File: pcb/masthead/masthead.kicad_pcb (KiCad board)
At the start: 2 copper layers, 48.6 x 56.5 mm, 12 parts, among them J1 Screw_Terminal_01x01, J2 Screw_Terminal_01x01, J3 VEML7700, SW1 TILT, U1 TSR_1-2450, U2 WeMos_mini, U3 BMP581

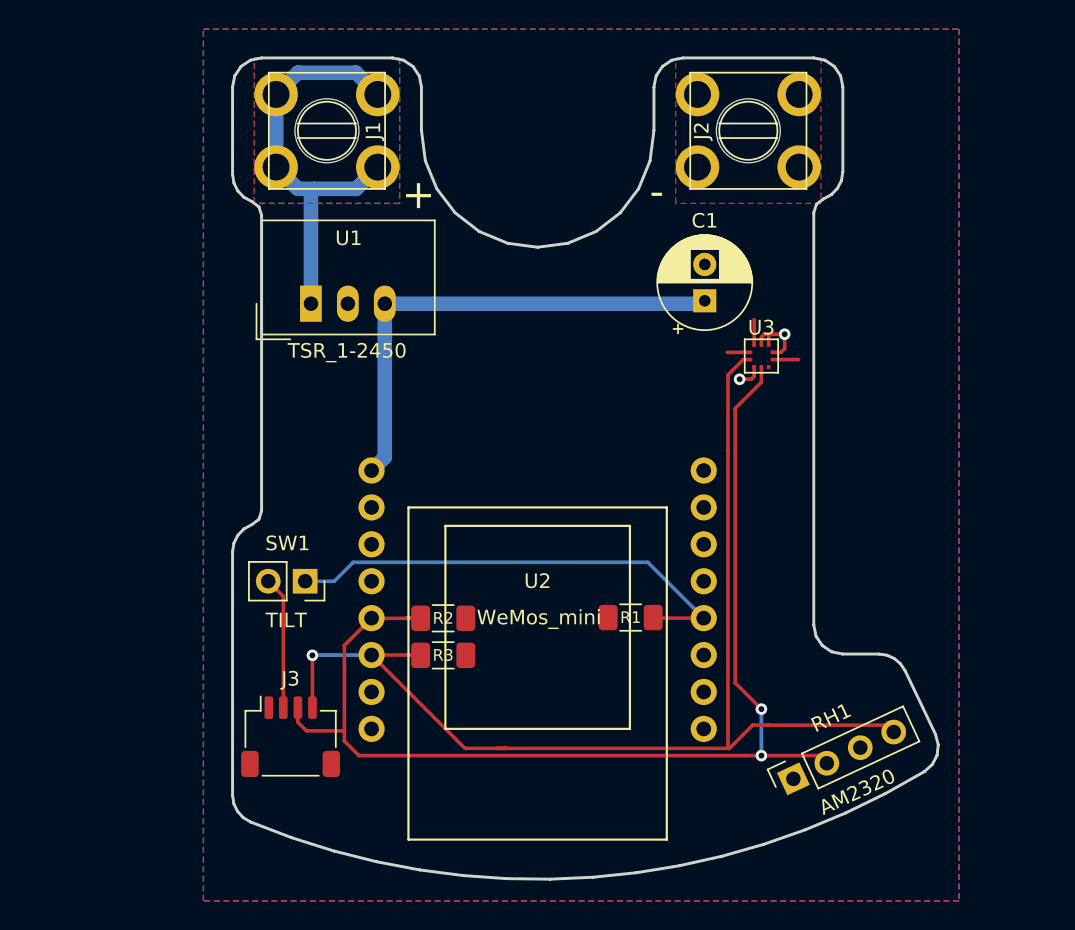
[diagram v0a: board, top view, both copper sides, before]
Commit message: Tweaks
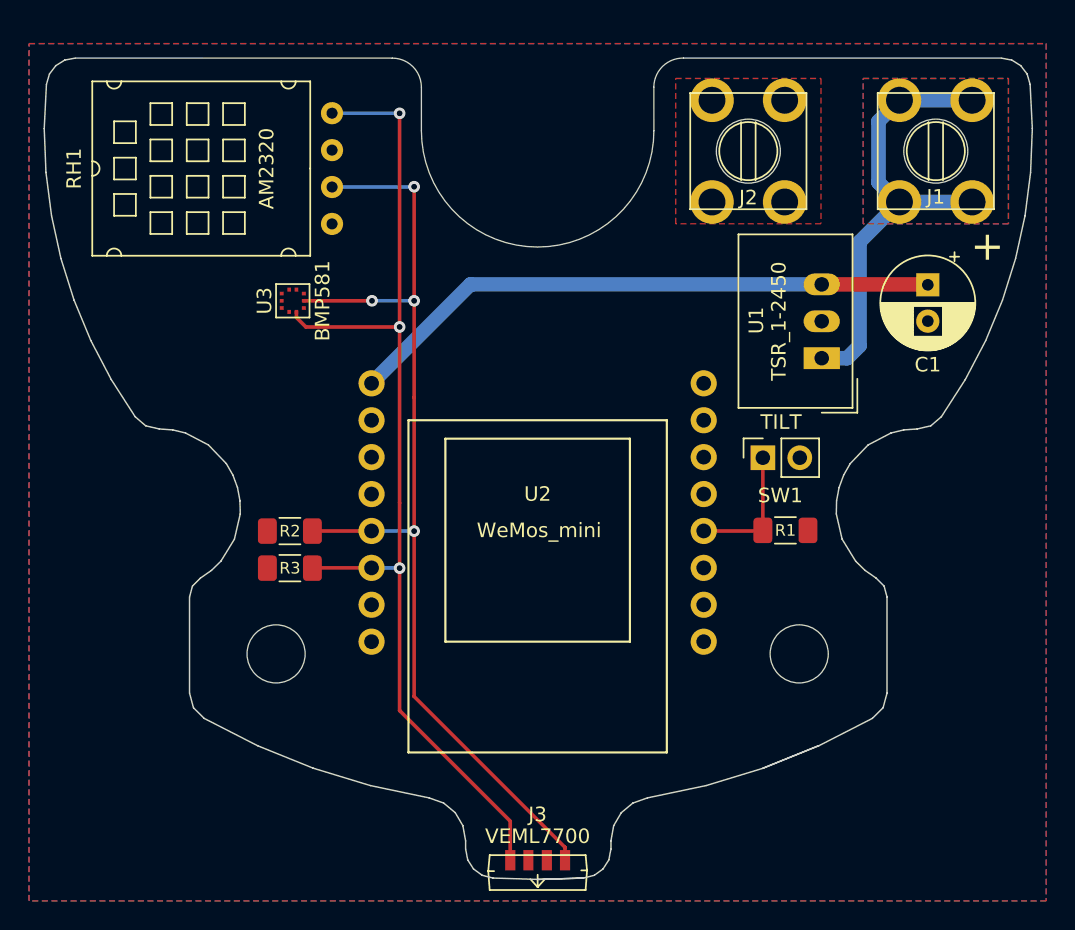
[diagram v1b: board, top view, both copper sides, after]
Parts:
- J1, J2: value Screw_Terminal_01x01 -> Open screw terminal 5x7
- J3: footprint Connector_JST:JST_SH_SM04B-SRSS-TB_1x04-1MP_P1.00mm_Horizontal -> PDJR_Module:VEML7700_SIDE
- RH1: footprint Connector_PinSocket_2.54mm:PinSocket_1x04_P2.54mm_Vertical -> PDJR_Sensor:AM2320_HORIZ
- moved RH1 52.7 mm to (-14.2, 2.60), turned to 90 degrees
- moved J1 41.9 mm to (27.4, 1.40), turned to 90 degrees
- moved U1 35.3 mm to (19.6, 15.7), turned to 90 degrees
- moved SW1 32.6 mm to (15.5, 22.5), turned to 90 degrees
- moved U3 32.5 mm to (-16.9, 11.7), turned to 90 degrees
- moved J3 19.0 mm to (0.00, 50.2)
- moved C1 15.4 mm to (26.9, 10.6), turned to 270 degrees
- moved R1 12.2 mm to (17.1, 27.5), turned to 180 degrees
- moved R3 12.1 mm to (-17.1, 30.1), turned to 0 degrees
- moved R2 12.1 mm to (-17.1, 27.6), turned to 0 degrees
- moved U2 6.00 mm to (0.00, 25.0)
- moved J2 1.40 mm to (14.5, 1.40), turned to 270 degrees
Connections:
- J3 pad 1: +3V3 -> /SCL
- J3 pad 2: GND -> +3V3
- J3 pad 3: Net-(J3-Pad3) -> GND
- J3 pad 4: Net-(J3-Pad4) -> /SDA
- R2 pad 2: Net-(J3-Pad3) -> /SDA
- R3 pad 2: Net-(J3-Pad4) -> /SCL
- RH1 pad 2: Net-(J3-Pad3) -> /SDA
- RH1 pad 4: Net-(J3-Pad4) -> /SCL
- U2 pad 5: Net-(J3-Pad3) -> /SDA
- U2 pad 6: Net-(J3-Pad4) -> /SCL
- U3 pad 2: Net-(J3-Pad4) -> /SCL
- U3 pad 4: Net-(J3-Pad3) -> /SDA
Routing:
- net Net-(J3-Pad3): track 80.2 -> 0.00 mm, vias 2 -> 0
- net Net-(J3-Pad4): track 78.8 -> 0.00 mm, vias 1 -> 0
- net /SCL: track 0.00 -> 73.0 mm, vias 0 -> 3
- net /SDA: track 0.00 -> 70.9 mm, vias 0 -> 4
- net Net-(R1-Pad2): track 33.1 -> 9.09 mm
- net GND: track 15.8 -> 0.00 mm, vias 2 -> 0
- net +5V: track 34.0 -> 41.1 mm
- net +3V3: track 5.11 -> 0.00 mm
- net Net-(J1-Pad1): track 29.5 -> 32.3 mm
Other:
- board size 48.6 x 56.5 mm -> 68 x 56.5 mm
- board text removed: "-"
